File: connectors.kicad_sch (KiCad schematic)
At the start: 4 parts, among them J1 0436500200, J2 0430450200, J3 0436500900, J4 0430451600

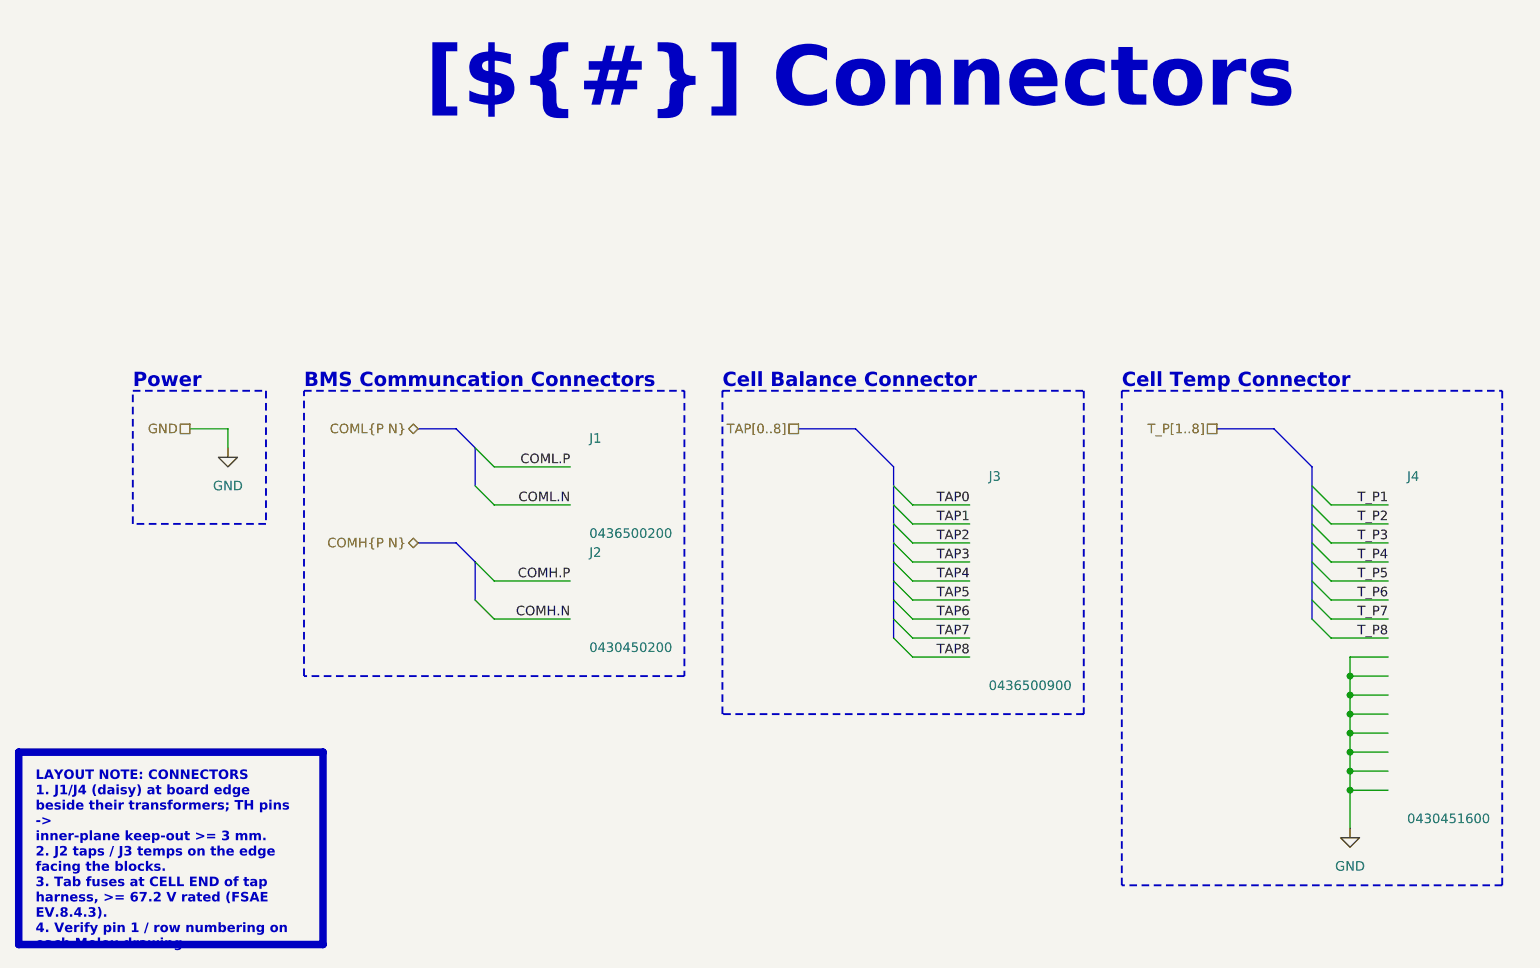
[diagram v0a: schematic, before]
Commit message: SCH[Cleaning]:Updated Connectors not sure still, added sprate bat and ground connections, updated commincation conncetors. PCB[Layout]:Inital layout of compents need to fit on board size once tap connecton method is decided.
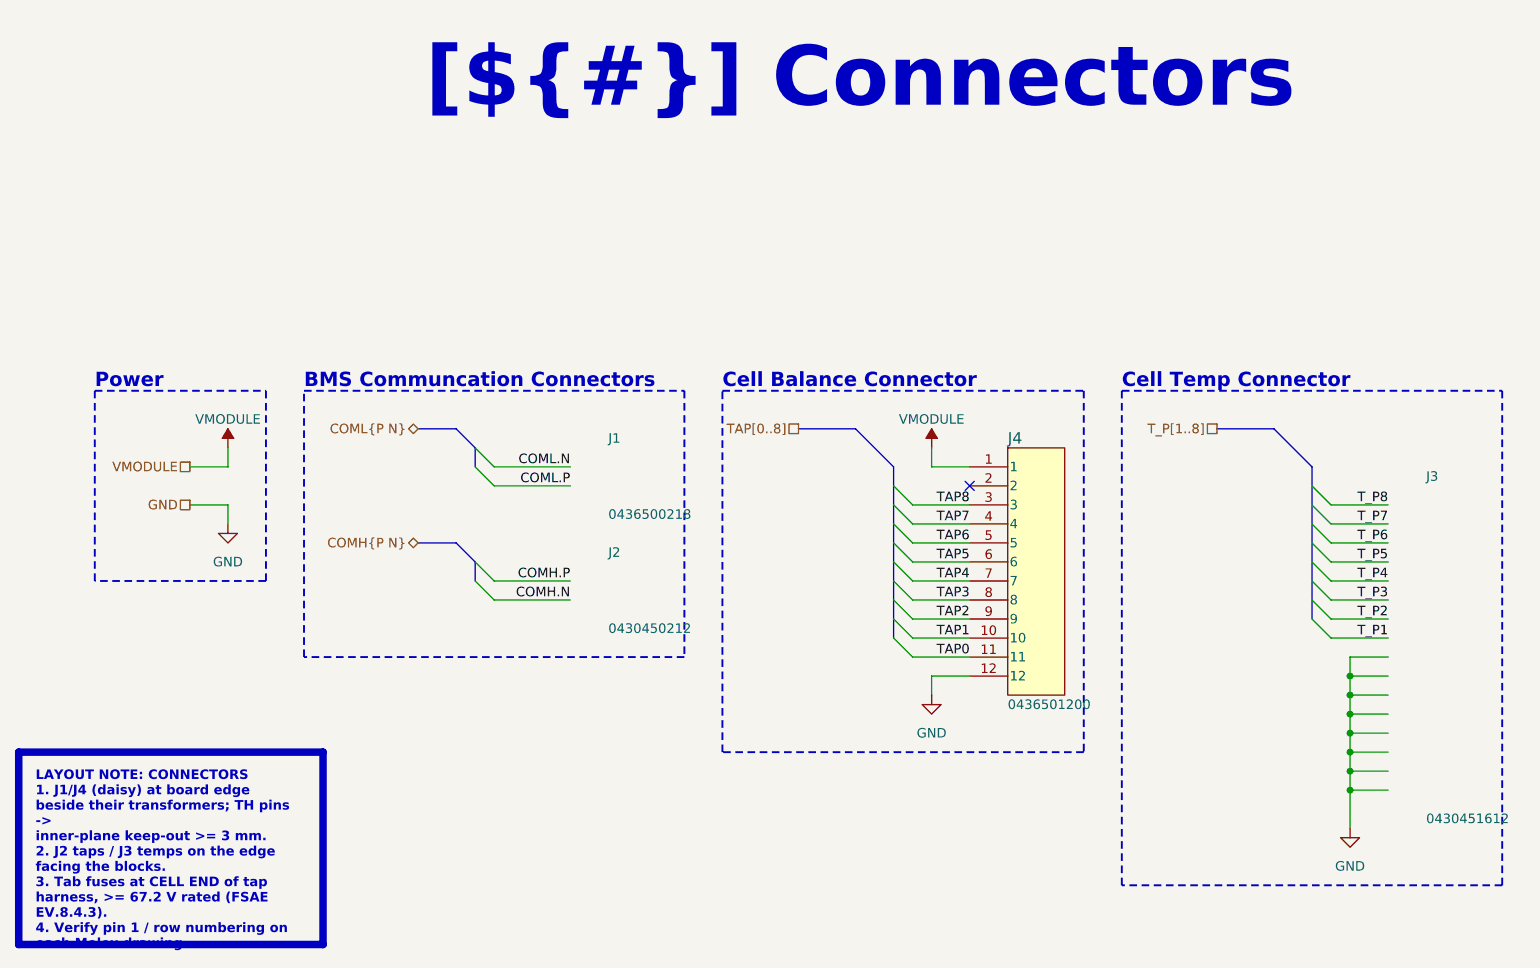
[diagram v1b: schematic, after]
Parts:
- removed J1: 0436500200, remote_0436500200:CONN_SD-43650-001_02_MOL, symbol remote_0436500200:0436500200
- removed J2: 0430450200, remote_0430450200:CONN_SD-43045-001_02_MOL, symbol remote_0430450200:0430450200
- removed J3: 0436500900, remote_0436500900:CONN_SD-43650-001_09_MOL, symbol remote_0436500900:0436500900
- removed J4: 0430451600, remote_0430451600:CONN_SD-43045-001_16_MOL, symbol remote_0430451600:0430451600
- added J1: 0436500218, remote_0436500218:CONN_SD-43650-007_02_MOL, symbol remote_0436500218:0436500218
- added J2: 0430450212, remote_0430450212:CONN_SD-43045-005_02_MOL, symbol remote_0430450212:0430450212
- added J3: 0430451612, remote_0430451612:CONN_SD-43045-005_16_MOL, symbol remote_0430451612:0430451612
- added J4: 0436501200, remote_0436501200:CONN_SD-43650-001_12_MOL, symbol remote_0430451200:0430451200
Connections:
- net COMH.N: now also J2.2
- net COMH.P: now also J2.1
- net COML.N: now also J1.1
- net COML.P: now also J1.2
- net GND: now also J3.10, J3.11, J3.12, J3.13, J3.14, J3.15, J3.16, J3.9, J4.12
- net TAP0: now also J4.11
- net TAP1: now also J4.10
- net TAP2: now also J4.9
- net TAP3: now also J4.8
- net TAP4: now also J4.7
- net TAP5: now also J4.6
- net TAP6: now also J4.5
- net TAP7: now also J4.4
- net TAP8: now also J4.3
- net T_P1: now also J3.8
- net T_P2: now also J3.7
- net T_P3: now also J3.6
- net T_P4: now also J3.5
- net T_P5: now also J3.4
- net T_P6: now also J3.3
- net T_P7: now also J3.2
- net T_P8: now also J3.1
- new net VMODULE: J4.1
- no-connect marks 0 -> 1
